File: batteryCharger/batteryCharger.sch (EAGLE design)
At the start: 71 parts, among them J1 B4P-VH(LF)(SN), Q1 SIR414DP-T1-GE3, Q2 SI7635DP-T1-GE3, Q3 SI7635DP-T1-GE3, Q4 SIR414DP-T1-GE3, Q5 SI7635DP-T1-GE3

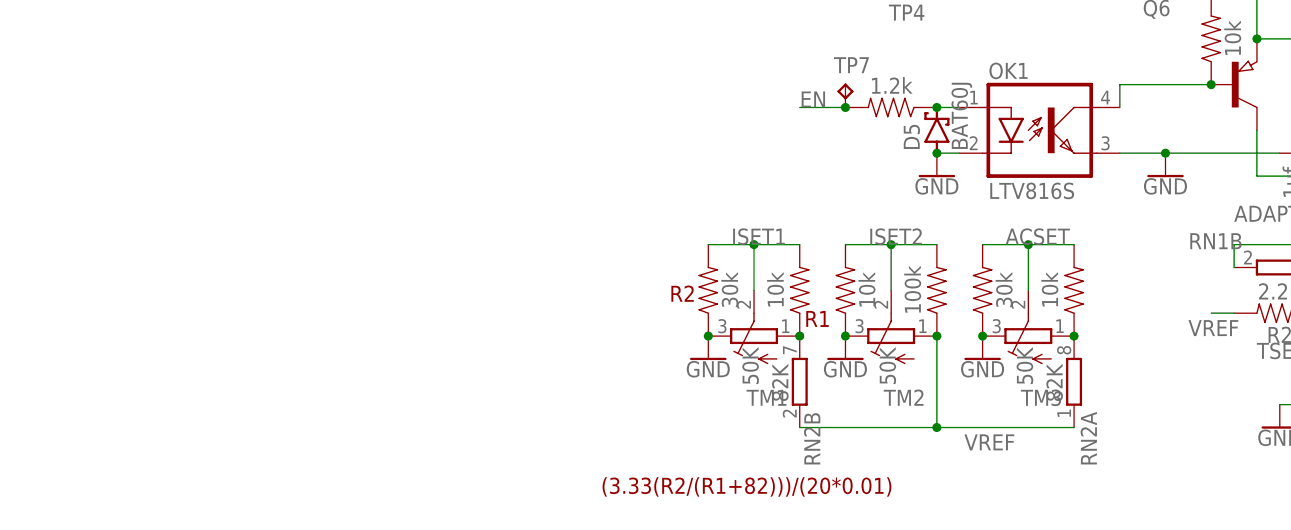
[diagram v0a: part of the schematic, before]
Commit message: final board file
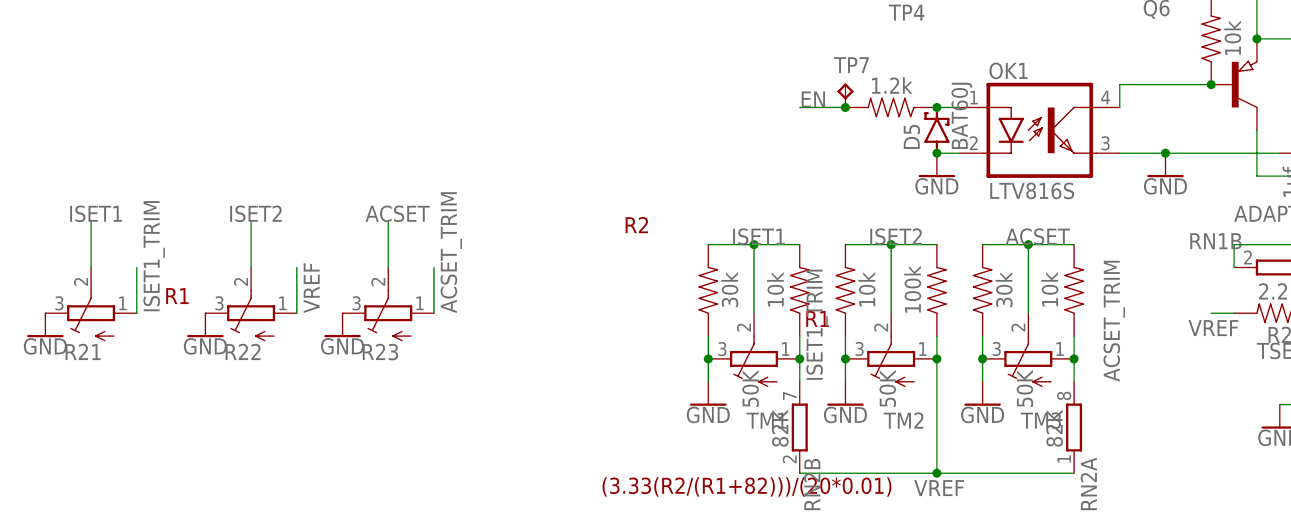
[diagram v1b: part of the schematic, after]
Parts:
- added R21, R22, R23: (no value), pot:TRIM_EU-3223W
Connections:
- removed net N$11: R5.1, RN2B.2, TM1.A
- removed net N$9: R19.1, RN2A.2, TM3.A
- new net ACSET_TRIM: R19.1, R23.A, RN2A.2, TM3.A
- new net ISET1_TRIM: R21.A, R5.1, RN2B.2, TM1.A
- net ACSET: now also R23.S
- net GND: now also R21.E, R22.E, R23.E
- net ISET1: now also R21.S
- net ISET2: now also R22.S
- net VREF: now also R22.A
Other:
- moved on the sheet: RN2A, RN2B, TM1, TM2, TM3
